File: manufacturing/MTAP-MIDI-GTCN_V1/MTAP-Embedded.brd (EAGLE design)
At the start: 27.9 x 62.9 mm, 54 parts, among them IC1 ESP32-WROOM-32UE-N8, IC2 AMS1117-3.3, IC3 PCM1821IRTER, J1 629105150521

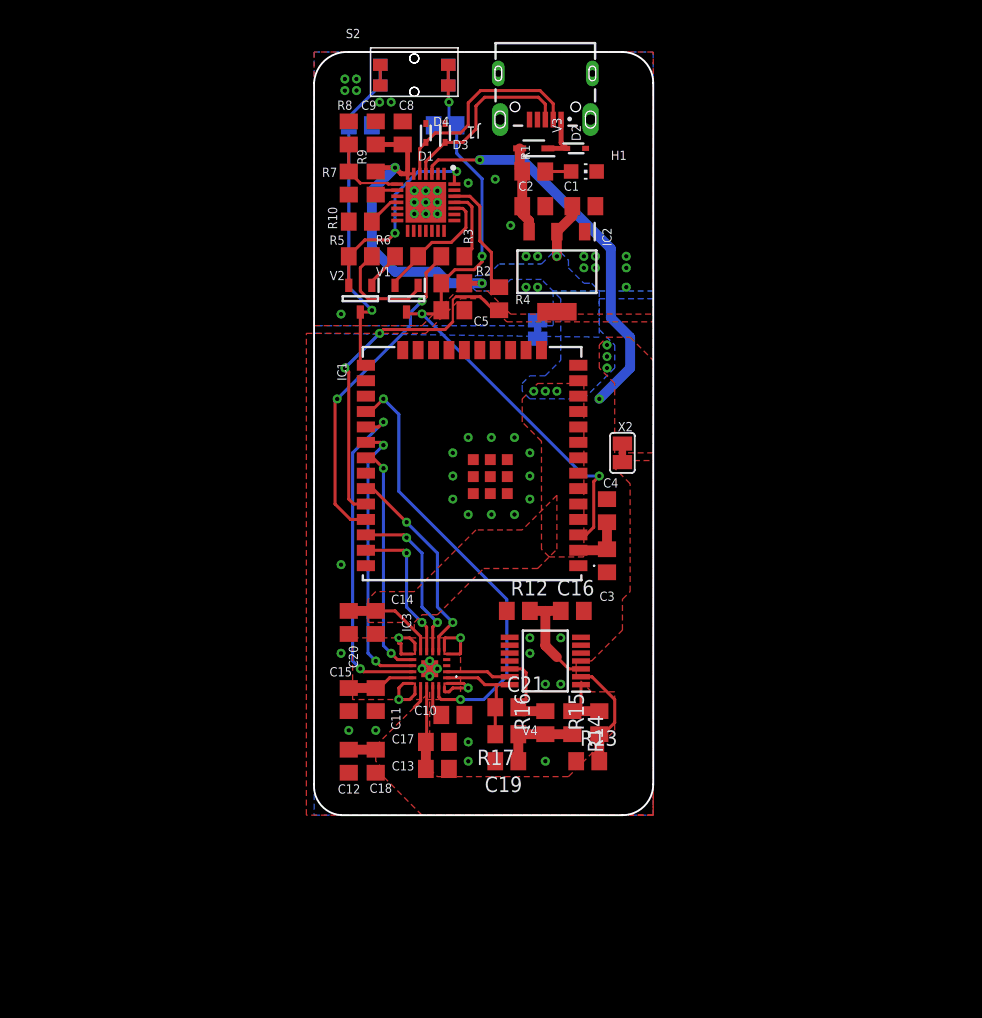
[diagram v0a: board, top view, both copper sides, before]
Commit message: New Layout
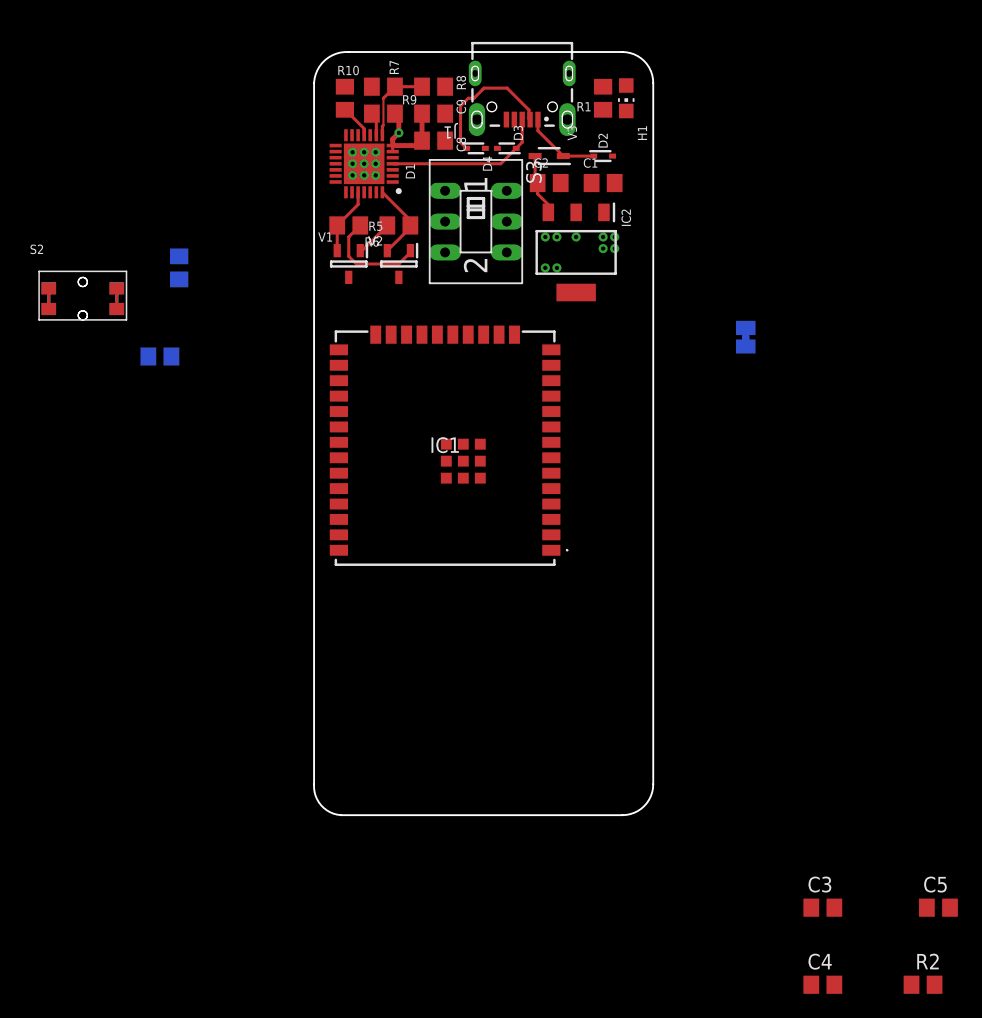
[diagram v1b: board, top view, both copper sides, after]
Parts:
- removed C10, C12: 1u, rcl_GruS:C0805
- removed C11, C13, C14: 10u, rcl_GruS:C0805
- removed C15, C17, C18, C20: 100n, rcl_GruS:C0805
- removed C16, C21: 10n, rcl_GruS:C0805
- removed C19: 680n, rcl_GruS:C0805
- removed IC3: PCM1821IRTER, adc-dac_GruS:WQFN20
- removed R12: 6k2, rcl_GruS:R0805
- removed R13: 2k4, rcl_GruS:R0805
- removed R14: 240, rcl_GruS:R0805
- removed R15: 5k1, rcl_GruS:R0805
- removed R16: 200, rcl_GruS:R0805
- removed R17: 750, rcl_GruS:R0805
- removed R3, R4: 0R, rcl_GruS:R0805
- removed V4: TLV9354IPWR, opv_GruS:SOP65P640X120-14N
- removed X2: (no value), con_GruS:MYLIB_SJ-SHORT
- added S3: (no value), switch_GruS:A68-A31
- moved R2 69.6 mm to (50.2, -14.0)
- moved C5 63.4 mm to (51.4, -7.62)
- moved C4 42.9 mm to (41.9, -14.0), turned to 0 degrees
- moved C3 33.7 mm to (41.9, -7.62), turned to 0 degrees
- moved S1 32.9 mm to (-19.1, 42.5)
- moved S2 32.9 mm to (-19.1, 42.5)
- moved C6 25.2 mm to (-12.7, 37.8)
- moved C7 24.9 mm to (-11.1, 45.1), turned to 90 degrees
- moved R11 17.2 mm to (35.6, 39.4)
- moved R10 10.2 mm to (2.54, 59.1), turned to 270 degrees
- moved R7 8.44 mm to (5.71, 60.0), turned to 0 degrees
- moved R1 8.31 mm to (23.8, 59.1), turned to 270 degrees
- moved R8 7.96 mm to (9.84, 60.0), turned to 180 degrees
- moved H1 6.97 mm to (25.7, 59.1), turned to 180 degrees
- moved D1 5.99 mm to (4.13, 53.7), turned to 180 degrees
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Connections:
- removed net AVDD: C12.1, C18.1, IC3.16, V4.4, X2.2
- removed net IN1P: C21.1, IC3.1, R17.2, V4.14
- removed net IN2M: IC3.4
- removed net IN2P: IC3.3
- removed net N$10: R14.1, R15.2, V4.1
- removed net N$11: C21.2, R16.2, V4.12
- removed net N$13: C11.1, C15.1, IC3.14
- removed net N$17: C13.1, C17.1, IC3.17
- removed net N$5: R12.1
- removed net N$6: C16.1, R12.2, V4.3
- removed net N$7: R13.2, R15.1, V4.2
- removed net N$8: C19.1, R14.2, R16.1, R17.1
- removed net N$9: C10.1, IC3.18
- new net RXD1: S3.6
- new net TXD1: S3.3
- net +3V3: no longer C14.1, C20.1, IC3.9, X2.1
- net BCLK: no longer IC3.7
- net FSYNC: no longer IC3.8
- net FTM0: no longer IC3.19
- net GND: no longer C10.2, C11.2, C12.2, C13.2, C14.2, C15.2, C16.2, C17.2, C18.2, C19.2, C20.2, IC3.10, IC3.15, IC3.2, IC3.20, IC3.21, IC3.22, IC3.23, IC3.24, IC3.25, IC3.5, R13.1, V4.10, V4.11, V4.13, V4.5, V4.6, V4.9
- net MD0: no longer IC3.12
- net MD1: no longer IC3.11
- net MSZ: no longer IC3.13
- net RXD: now also S3.2; no longer R3.2
- net RXD0: now also S3.4; no longer R4.1
- net SDATA: no longer IC3.6
- net TXD: now also S3.5; no longer R4.2
- net TXD0: now also S3.1; no longer R3.1
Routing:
- net GND: track 56.1 -> 0.00 mm, vias 34 -> 0
- net EN: track 52.9 -> 1.70 mm, vias 4 -> 0
- net +3V3: track 44.8 -> 8.28 mm, vias 9 -> 2
- net FTM0: track 36.4 -> 0.00 mm, vias 2 -> 0
- net RXD0: track 29.2 -> 0.00 mm, vias 2 -> 0
- net MSZ: track 27.7 -> 0.00 mm, vias 2 -> 0
- net TXD0: track 27.1 -> 0.00 mm, vias 2 -> 0
- net GPIO0: track 27.9 -> 1.70 mm, vias 1 -> 0
- net MD0: track 23.3 -> 0.00 mm, vias 2 -> 0
- net MD1: track 19.3 -> 0.00 mm, vias 2 -> 0
- net SDATA: track 17.2 -> 0.00 mm, vias 2 -> 0
- net BCLK: track 14.1 -> 0.00 mm, vias 2 -> 0
- net FSYNC: track 12.3 -> 0.00 mm, vias 2 -> 0
- net DTR: track 17.2 -> 6.55 mm, vias 2 -> 0
- net TXD: track 9.76 -> 0.00 mm
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- removed copper zone on layer 1, net +3V3
- removed copper zone on layer 16, net +3V3
- removed copper zone on layer 1, net AVDD
- removed copper zone on layer 1, net GND
- removed copper zone on layer 16, net GND
- removed copper zone on layer 1, net PGND
- removed copper zone on layer 16, net PGND

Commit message: upd board
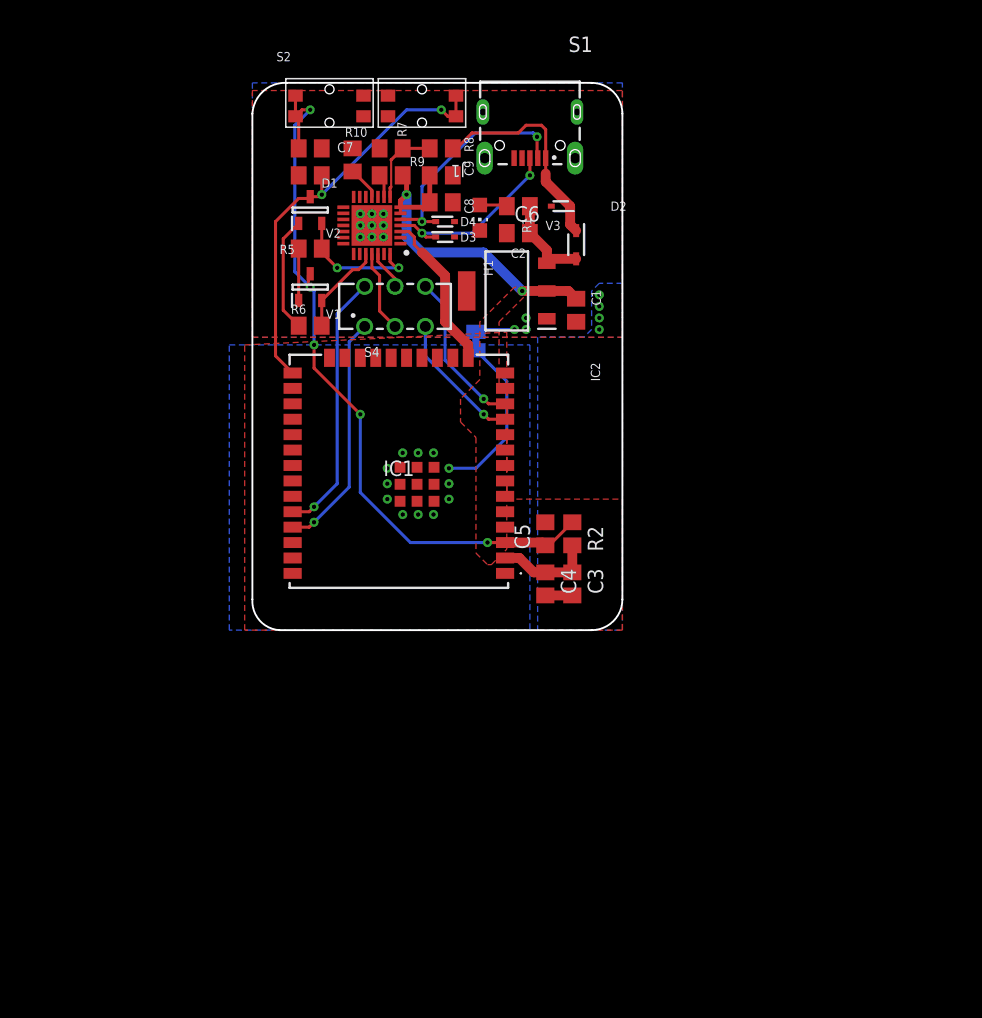
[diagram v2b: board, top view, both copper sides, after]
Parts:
- removed S3: (no value), switch_GruS:A68-A31
- added S4: (no value), switch_GruS:452404020202
- moved R2 47.1 mm to (21.3, 23.2), turned to 270 degrees
- moved C5 44.7 mm to (19.1, 23.2), turned to 90 degrees
- moved C4 40.2 mm to (19.1, 19.1), turned to 270 degrees
- moved C3 33.7 mm to (21.3, 19.1), turned to 270 degrees
- moved S1 32.1 mm to (8.89, 58.4), flipped to the top
- moved S2 25.8 mm to (1.27, 58.4)
- moved R11 22.2 mm to (13.3, 39.1)
- moved C6 19.4 mm to (-0.32, 52.7), flipped to the top
- moved H1 15.6 mm to (13.7, 49.2)
- moved C7 14.6 mm to (-0.32, 54.9), flipped to the top, turned to 0 degrees
- moved R1 11.3 mm to (16.8, 50.2), turned to 0 degrees
- moved C1 10.7 mm to (21.6, 41.6), turned to 270 degrees
- moved D3 8.90 mm to (10.8, 47.6), turned to 0 degrees
- moved R6 8.84 mm to (-0.32, 40.3), turned to 180 degrees
- moved V2 8.55 mm to (-0.32, 49.8), turned to 90 degrees
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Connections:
- removed net GPIO26: IC1.11
- removed net GPIO27: IC1.12
- net EN: now also S2.1, S2.2; no longer S2.3, S2.4
- net PGND: now also S2.3, S2.4; no longer S2.1, S2.2
- net RXD: now also S4.2; no longer S3.2
- net RXD0: now also S4.4; no longer S3.4
- net RXD1: now also IC1.12, S4.6; no longer S3.6
- net TXD: now also S4.5; no longer S3.5
- net TXD0: now also S4.1; no longer S3.1
- net TXD1: now also IC1.11, S4.3; no longer S3.3
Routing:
- net EN: track 1.70 -> 61.4 mm, vias 0 -> 5
- net GPIO0: track 1.70 -> 35.2 mm, vias 0 -> 2
- net GND: track 0.00 -> 29.6 mm, vias 0 -> 12
- net +3V3: track 8.28 -> 36.1 mm
- net RXD0: track 0.00 -> 21.8 mm, vias 0 -> 1
- net TXD0: track 0.00 -> 19.8 mm, vias 0 -> 1
- net RXD1: track 0.00 -> 13.2 mm, vias 0 -> 1
- net VBUS: track 6.38 -> 18.0 mm
- net TXD1: track 0.00 -> 11.2 mm, vias 0 -> 1
- net USB_DN: track 11.5 -> 19.1 mm, vias 0 -> 2
- net RXD: track 0.00 -> 6.76 mm
- net DTR: track 6.55 -> 10.8 mm, vias 0 -> 2
- net TXD: track 0.00 -> 3.25 mm
- net RTS: track 5.52 -> 8.33 mm
- net +5V: track 5.09 -> 7.84 mm
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- added copper zone on layer 1, net +3V3
- added copper zone on layer 16, net AGND
- added copper zone on layer 1, net GND
- added copper zone on layer 16, net GND
- added copper zone on layer 1, net PGND
- added copper zone on layer 16, net PGND
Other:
- board size 27.9 x 62.9 mm -> 30.5 x 45.1 mm
